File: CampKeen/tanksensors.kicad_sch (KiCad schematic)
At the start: 8 parts, among them Q54 2N7000, Q55 IRF9Z34NPBF, Q56 2N7000, Q57 IRF9Z34NPBF

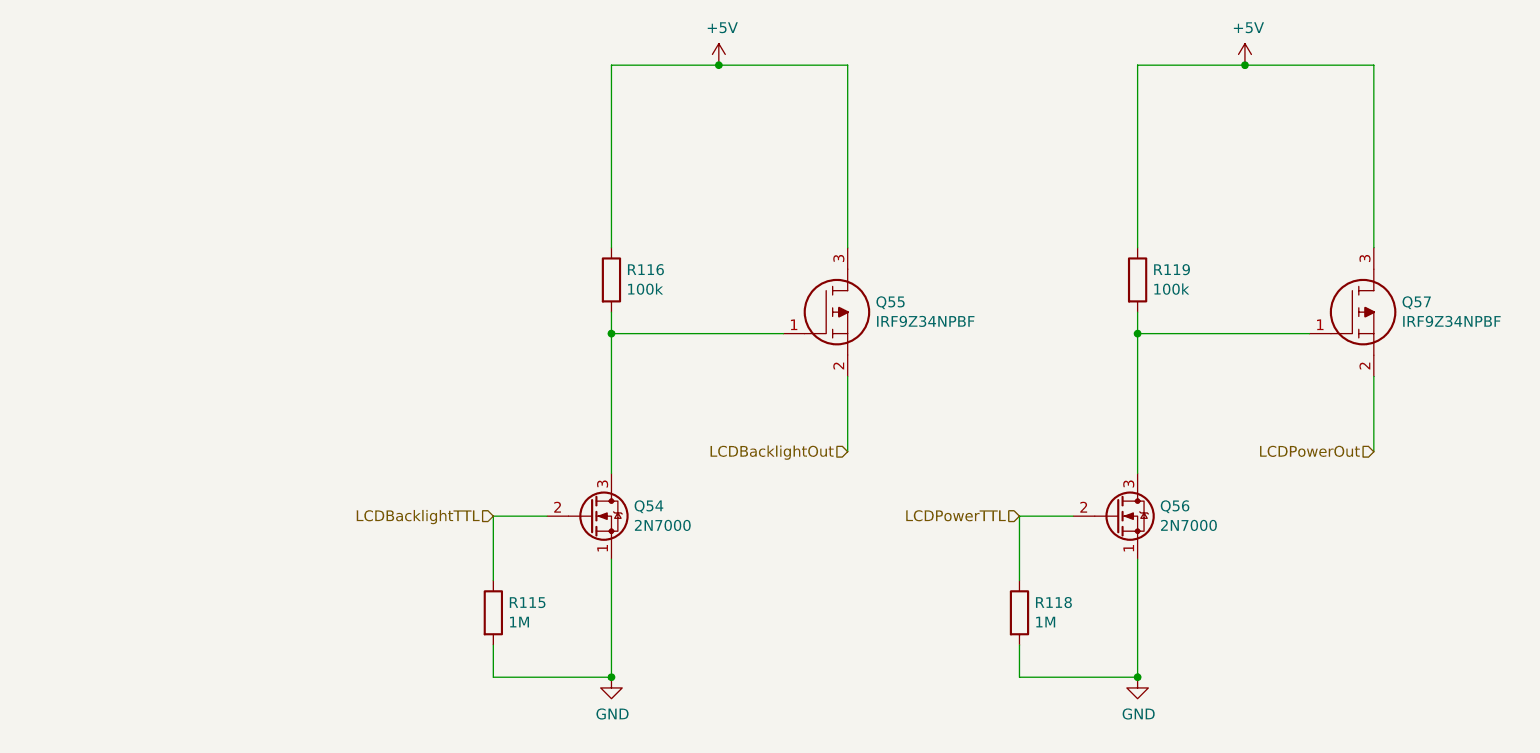
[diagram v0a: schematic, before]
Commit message: clean up of files
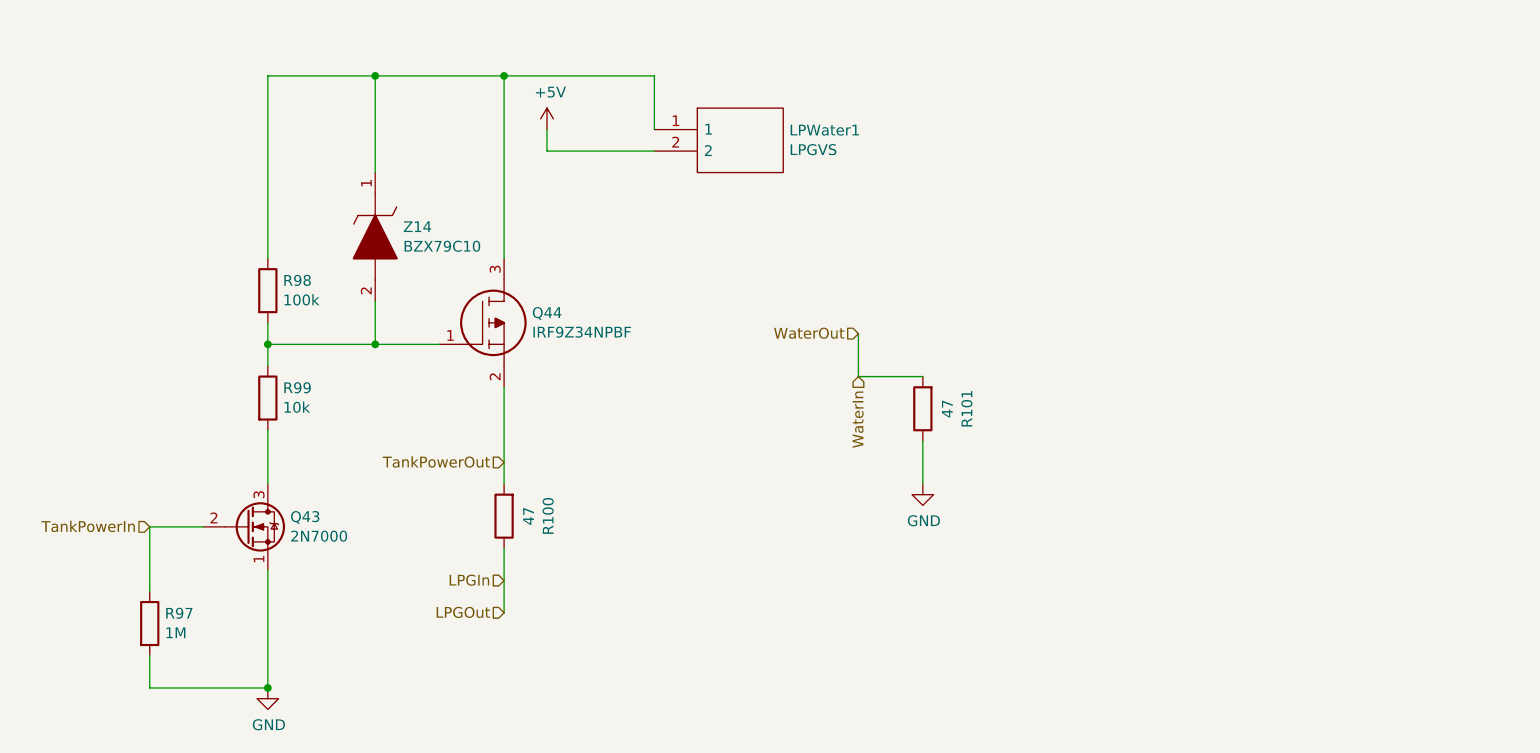
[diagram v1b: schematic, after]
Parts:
- removed Q54, Q56: 2N7000, Package_TO_SOT_THT:TO-92_Inline, symbol Transistor_FET:2N7000
- removed Q55, Q57: IRF9Z34NPBF, SamacSys_Parts:TO254P469X1042X1967-3P, symbol SamacSys_Parts:IRF9Z34NPBF
- removed R115, R118: 1M, Resistor_THT:R_Axial_DIN0207_L6.3mm_D2.5mm_P2.54mm_Vertical, symbol Device:R
- removed R116, R119: 100k, Resistor_THT:R_Axial_DIN0207_L6.3mm_D2.5mm_P2.54mm_Vertical, symbol Device:R
- added LPWater1: LPGVS, SamacSys_Parts:BK_HTC-15M, symbol SamacSys_Parts:BK_HTC-15M
- added Q43: 2N7000, Package_TO_SOT_THT:TO-92_Inline, symbol Transistor_FET:2N7000
- added Q44: IRF9Z34NPBF, SamacSys_Parts:TO254P469X1042X1967-3P, symbol SamacSys_Parts:IRF9Z34NPBF
- added R100, R101: 47, Resistor_THT:R_Axial_DIN0207_L6.3mm_D2.5mm_P2.54mm_Vertical, symbol Device:R
- added R97: 1M, Resistor_THT:R_Axial_DIN0207_L6.3mm_D2.5mm_P2.54mm_Vertical, symbol Device:R
- added R98: 100k, Resistor_THT:R_Axial_DIN0207_L6.3mm_D2.5mm_P2.54mm_Vertical, symbol Device:R
- added R99: 10k, Resistor_THT:R_Axial_DIN0207_L6.3mm_D2.5mm_P2.54mm_Vertical, symbol Device:R
- added Z14: BZX79C10, SamacSys_Parts:DIOAD1068W53L380D172, symbol SamacSys_Parts:BZX79C10
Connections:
- net +5V: now also LPWater1.2
- net GND: now also Q43.1 (S), R101.1, R97.2
- new net: LPWater1.1, Q44.3, R98.1, Z14.1
- new net: Q44.1, R98.2, R99.1, Z14.2
- new net: Q43.3 (D), R99.2
- new net LPGIn: R100.1
- new net TankPowerIn: Q43.2 (G), R97.1
- new net TankPowerOut: Q44.2, R100.2
- new net WaterIn: R101.2
